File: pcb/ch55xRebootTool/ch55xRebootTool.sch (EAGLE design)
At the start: 21 parts, among them IC1 CH443K, IC2 CH443K, U2 CH552G

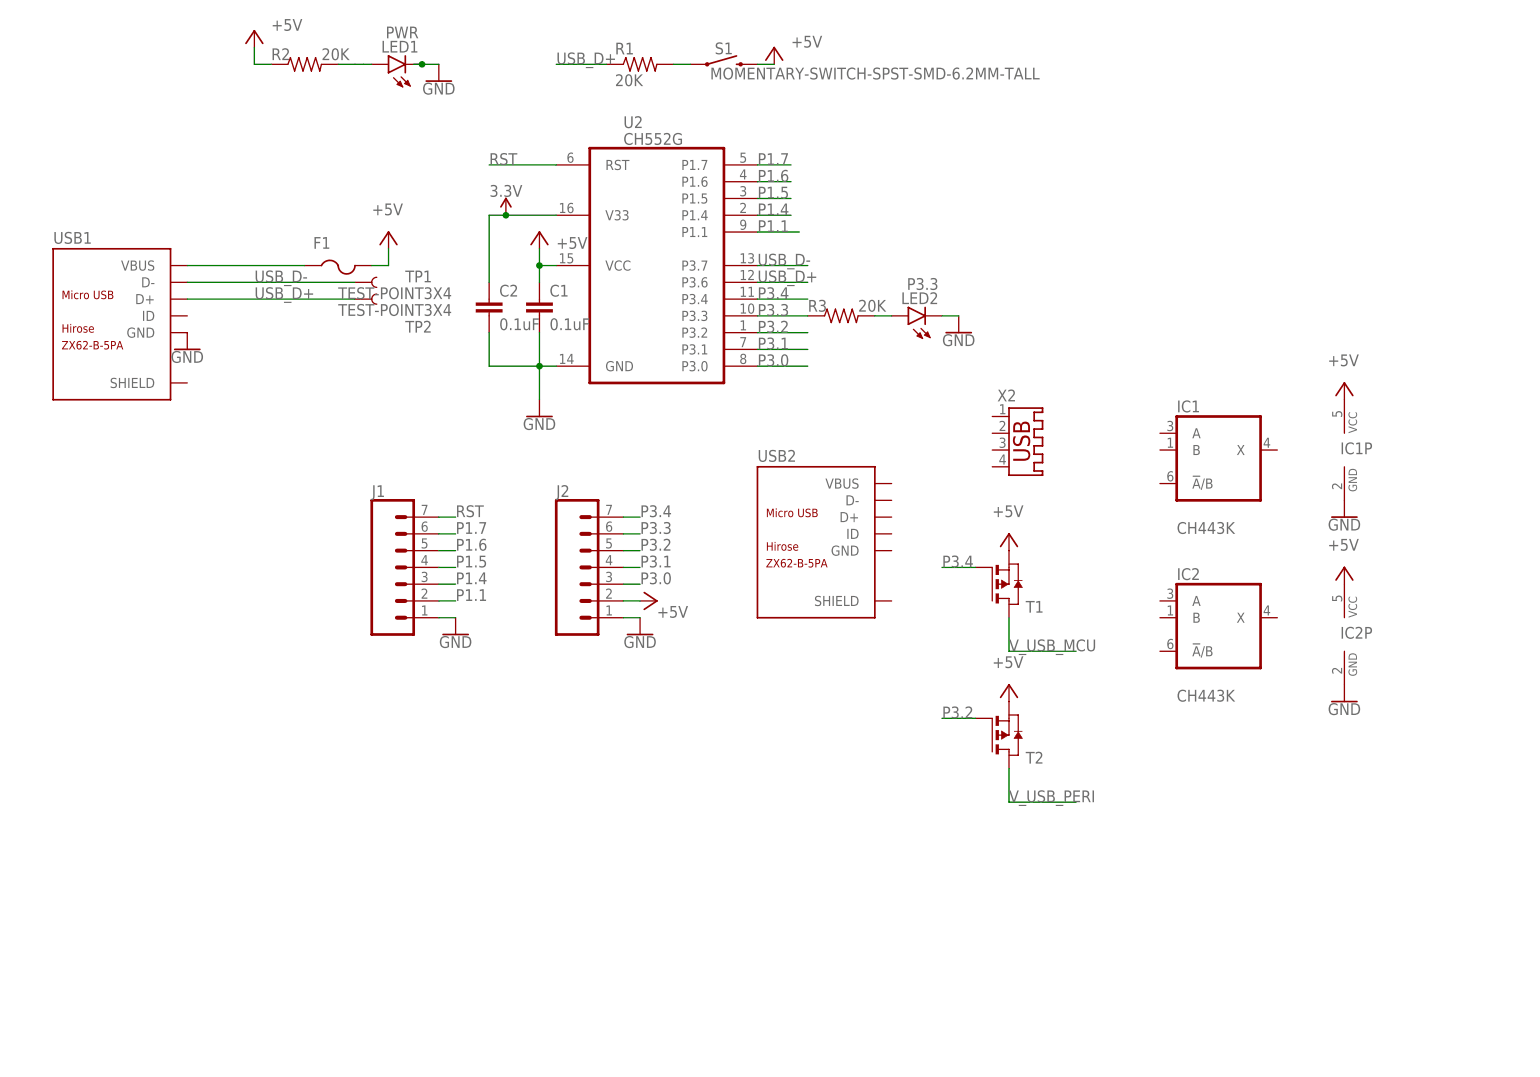
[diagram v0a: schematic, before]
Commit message: update board
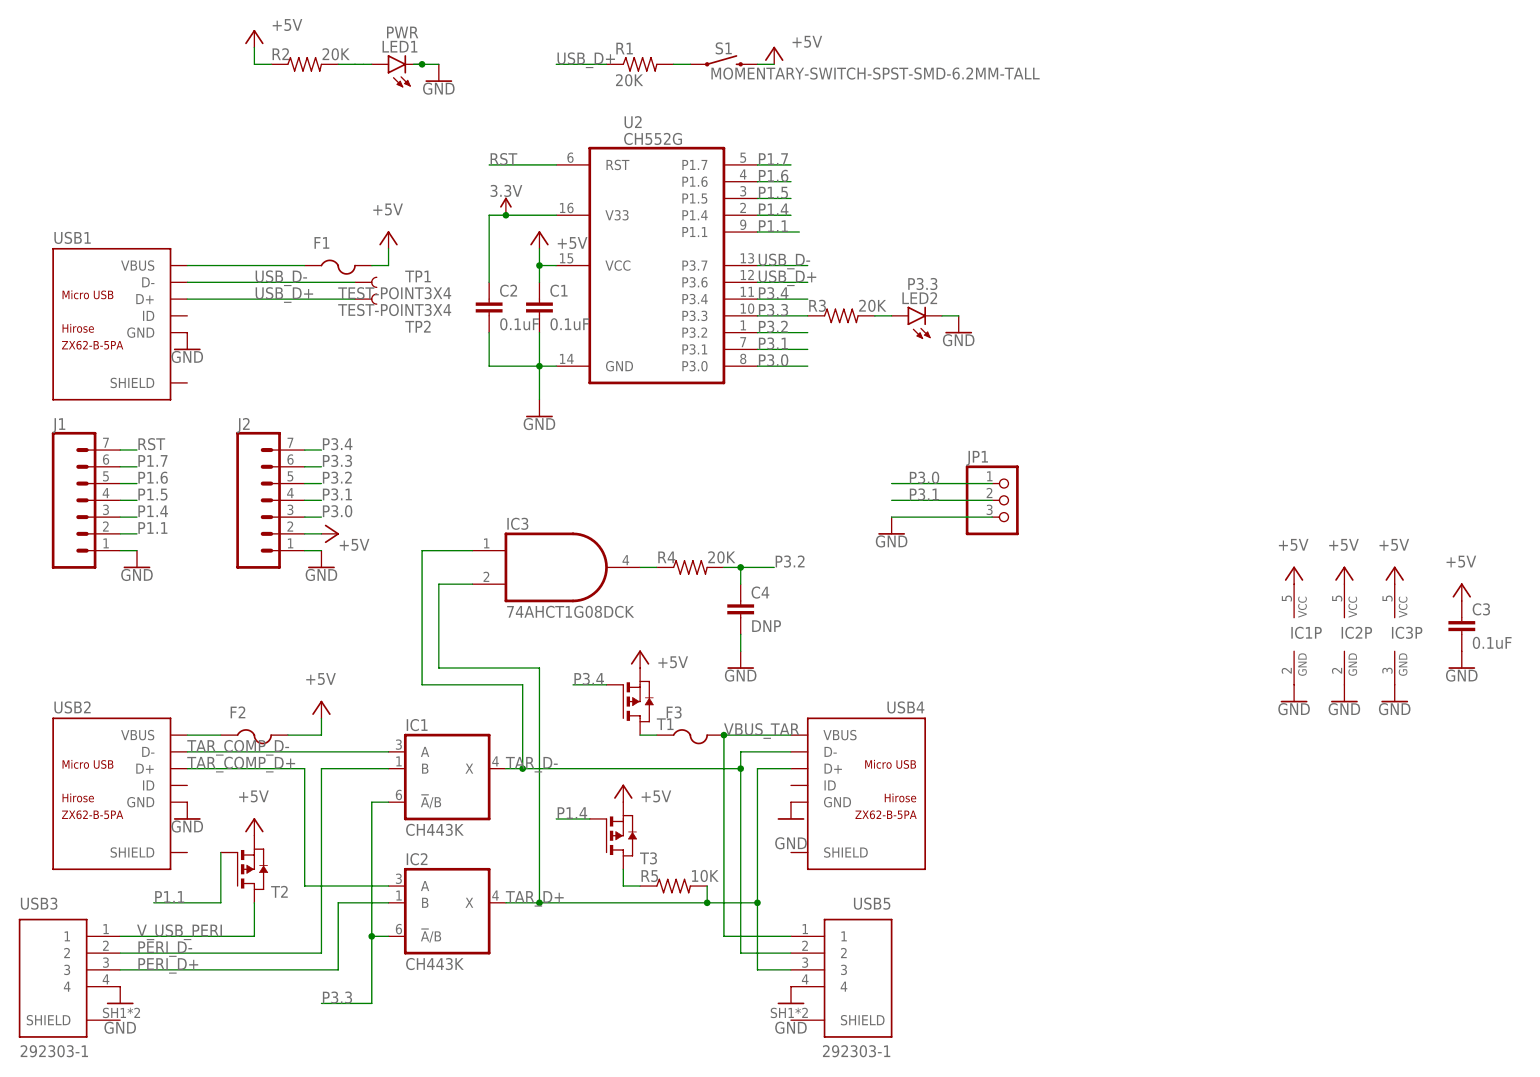
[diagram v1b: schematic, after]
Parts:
- removed X2: (no value), con-yamaichi:USB-A003
- added C3: 0.1uF, rcl:C-EUC0805K
- added C4: DNP, rcl:C-EUC0805K
- added F2, F3: (no value), adafruit:PTCFUSE-1206
- added IC3: 74AHCT1G08DCK, 74xx-little-us:74AHCT1G08DCK
- added JP1: (no value), pinhead:PINHD-1X3
- added R4: 20K, rcl:R-US_R0805
- added R5: 10K, rcl:R-US_R0805
- added T3: (no value), zetex:PMOSSOT23
- added USB3, USB5: 292303-1, USB connector:292303-1
- added USB4: ZX62-B-5PA, microusbConnector:MICRO-USB-SMD(ZX62-B-5PA)
- IC1, IC2: LCSC (none) -> C125185
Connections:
- removed net V_USB_MCU: T1.D
- new net N$4: IC3A.O, R4.1
- new net N$5: F3.1, T1.D
- new net N$7: R5.1, T3.D
- new net PERI_D+: IC2G$1.B, USB3.3
- new net PERI_D-: IC1G$1.B, USB3.2
- new net TAR_COMP_D+: IC2G$1.A, USB2.D+
- new net TAR_COMP_D-: IC1G$1.A, USB2.D-
- new net TAR_D+: IC2G$1.X, IC3A.I1, R5.2, USB4.D+, USB5.3
- new net TAR_D-: IC1G$1.X, IC3A.I0, USB4.D-, USB5.2
- new net VBUS_COMP: F2.1, USB2.VBUS
- new net VBUS_TAR: F3.2, USB4.VBUS, USB5.1
- net +5V: now also C3.1, F2.2, IC3P.VCC, T3.S
- net GND: now also C3.2, C4.2, IC3P.GND, JP1.3, USB2.GND, USB3.4, USB4.GND, USB5.4
- net P1.1: now also T2.G
- net P1.4: now also T3.G
- net P3.0: now also JP1.1
- net P3.1: now also JP1.2
- net P3.2: now also C4.1, R4.2; no longer T2.G
- net P3.3: now also IC1G$1.!A!/B, IC2G$1.!A!/B
- net V_USB_PERI: now also USB3.1
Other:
- moved on the sheet: IC1, IC1P, IC2, J1, J2, T1, T2, USB2
